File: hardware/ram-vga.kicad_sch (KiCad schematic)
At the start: 63 parts, among them J11 GPCO, J6 DB15_Female_HighDensity, J7 Conn_01x12_Male, U10 74HC245, U11 74HC245, U12 74HC109, U14 74HC04, U16 62256, U17 74HC00, U18 w27C512, U19 74LS161, U20 74HC165, U21 74HC00, U6 74HC590, U7 74HC590, U8 74HC32, Y1 16Mhz

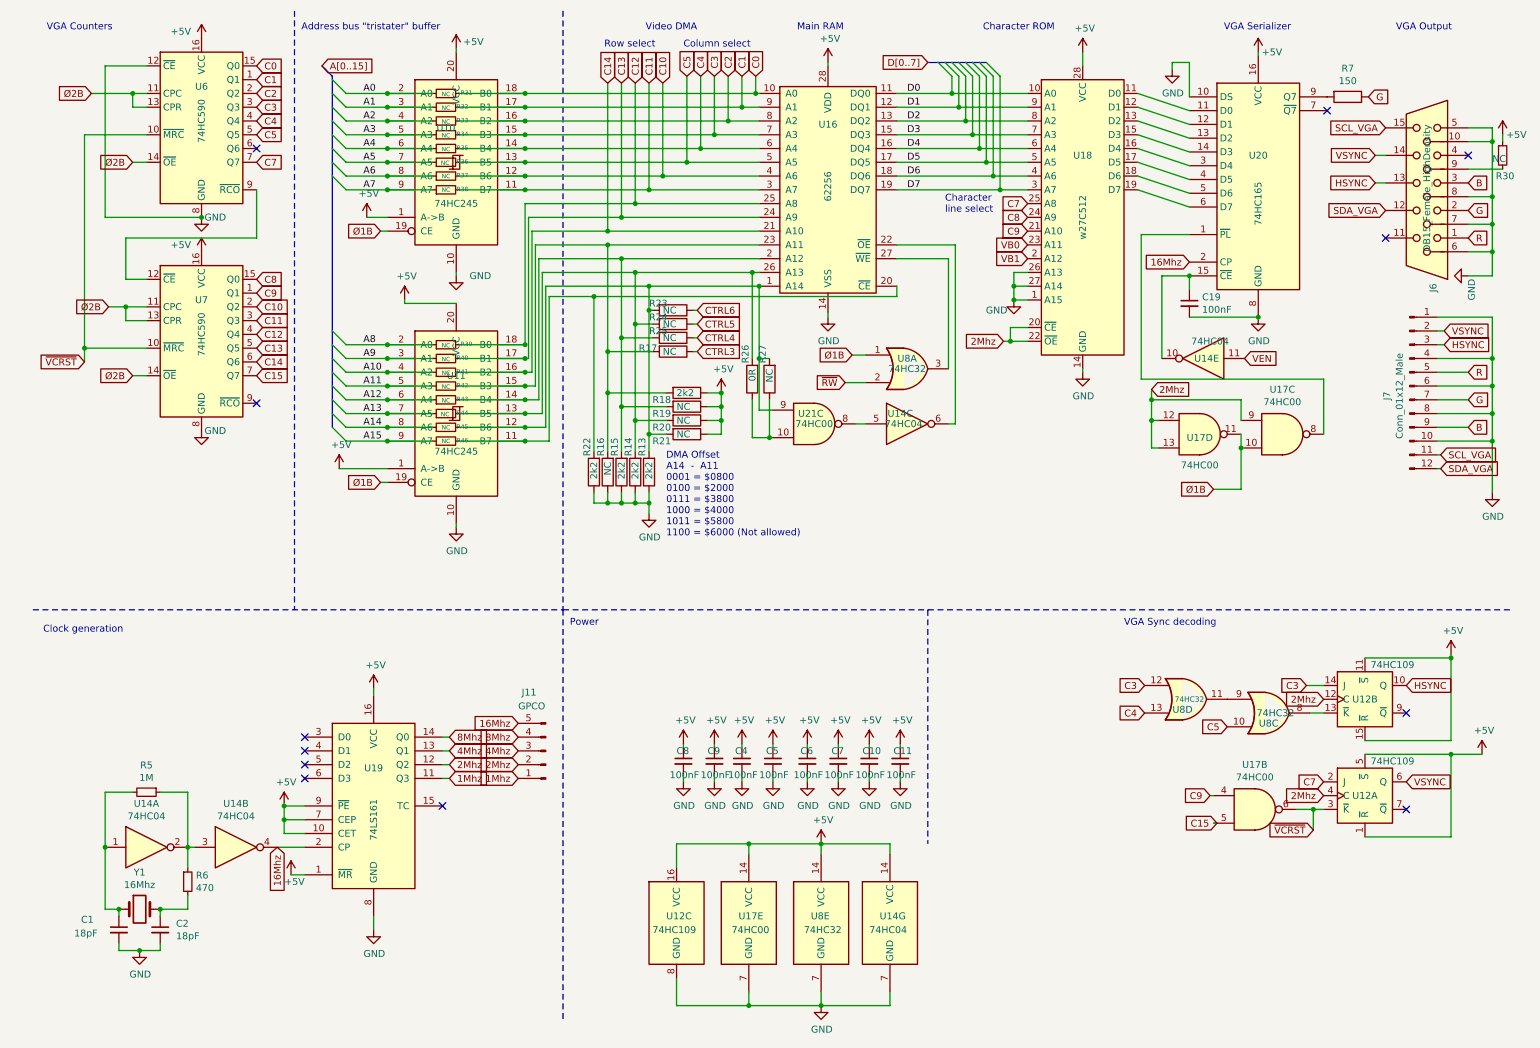
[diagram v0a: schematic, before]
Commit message: Revision 2 published
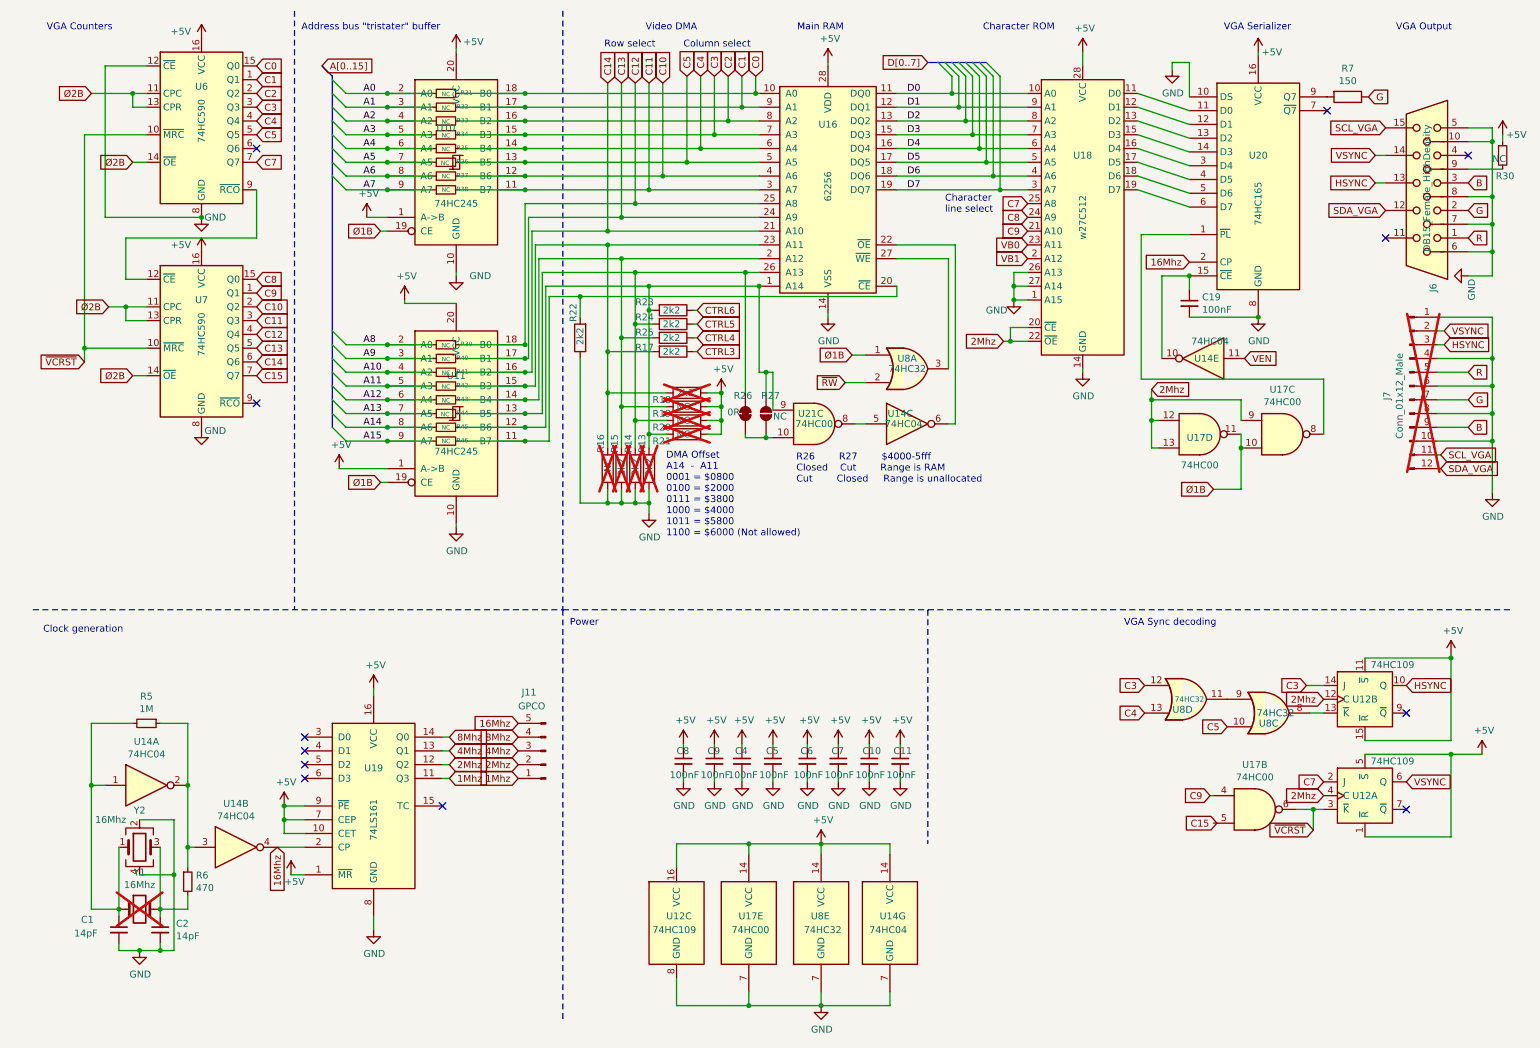
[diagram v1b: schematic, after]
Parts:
- added Y2: 16Mhz, Crystal:Crystal_SMD_3225-4Pin_3.2x2.5mm, symbol Device:Crystal_GND24
- C1, C2: value 18pF -> 14pF; LCSC (none) -> C519919
- C10, C11, C19, C4, C5, C6, C7, C8, C9: LCSC (none) -> C14663
- J6: footprint Connector_Dsub:DSUB-15-HD_Female_Horizontal_P2.29x2.54mm_EdgePinOffset9.40mm-Mountingholes -> Connector_Dsub:DSUB-15-HD_Female_Horizontal_P2.29x1.98mm_EdgePinOffset8.35mm_Housed_MountingHolesOffset10.89mm; LCSC (none) -> C138387
- J7, R16, R19, R20, R21, Y1: now not fitted
- R13, R14, R15, R18: LCSC (none) -> C114561; now not fitted
- R17, R23, R24, R25: value NC -> 2k2; LCSC (none) -> C114561
- R22: LCSC (none) -> C114561
- R26: footprint Jumper:SolderJumper-2_P1.3mm_Open_RoundedPad1.0x1.5mm -> Jumper:SolderJumper-2_P1.3mm_Bridged_RoundedPad1.0x1.5mm; symbol Device:R -> Jumper:SolderJumper_2_Bridged; now left out of the parts list
- R27: symbol Device:R -> Jumper:SolderJumper_2_Open; now left out of the parts list
- R5: LCSC (none) -> C17514
- R6: LCSC (none) -> C17710
- R7: LCSC (none) -> C17471
- U10, U11: LCSC (none) -> C72118
- U12, U19, U20, U6, U7: LCSC (none) -> C72115
- U14, U17, U21, U8: LCSC (none) -> C2325
- U16, U18: LCSC (none) -> C72121
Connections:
- net GND: now also Y2.2, Y2.4
- net at C1.1, R5.2, U14.1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: now also Y2.1
- net at C2.1, R6.2, Y1.2: now also Y2.3
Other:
- note added: "R26 R27 $4000-5fff Closed Cut Range is RAM Cut Closed Range is unallocated"
- moved on the sheet: R22, R5, U14A
